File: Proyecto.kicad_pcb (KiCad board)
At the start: 2 copper layers, 108.2 x 65.5 mm, 54 parts, among them P1 CONN_01X03, P2 CONN_01X03, Q1 BC808-40, Q2 BC808-40, U1 MCP2515, U2 MCP2551-I/SN, U3 AMS1117, U4 ACS712, U5 ACS712, U6 AMS1117

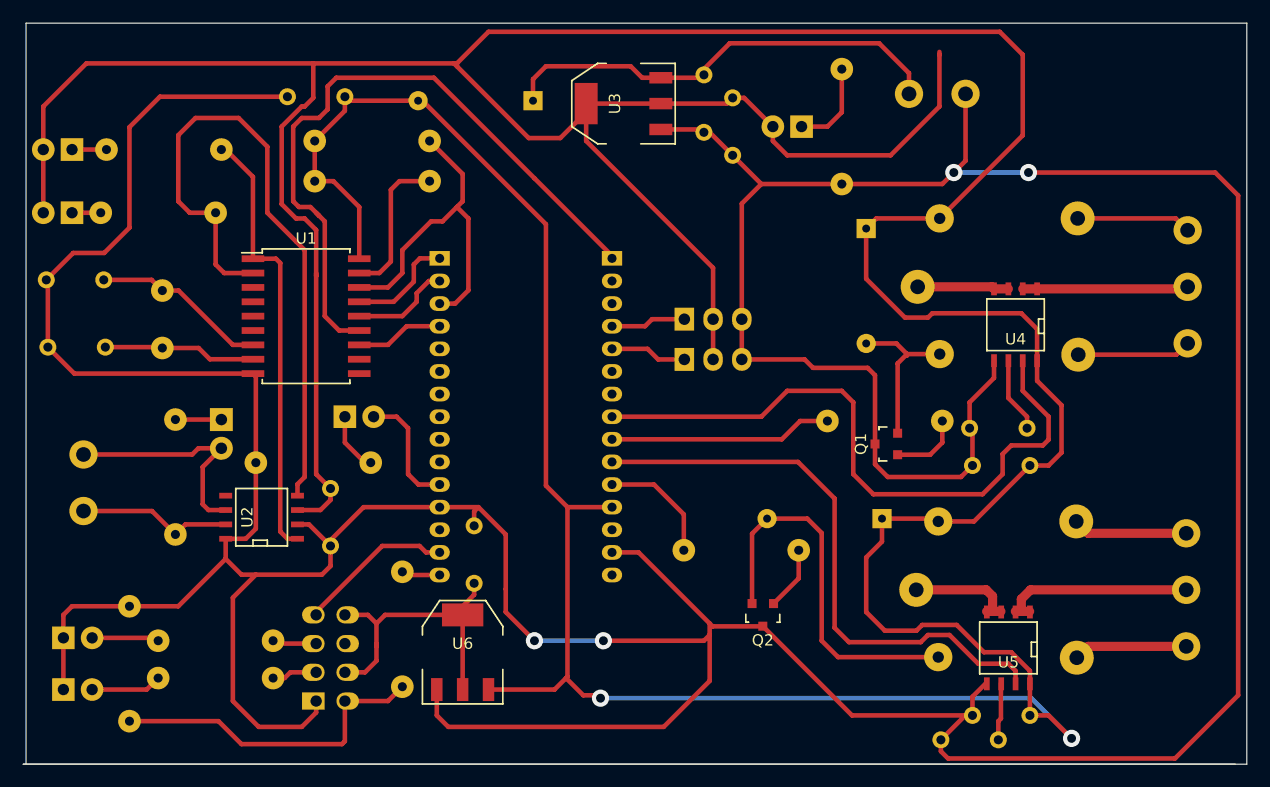
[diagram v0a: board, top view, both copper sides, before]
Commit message: fix
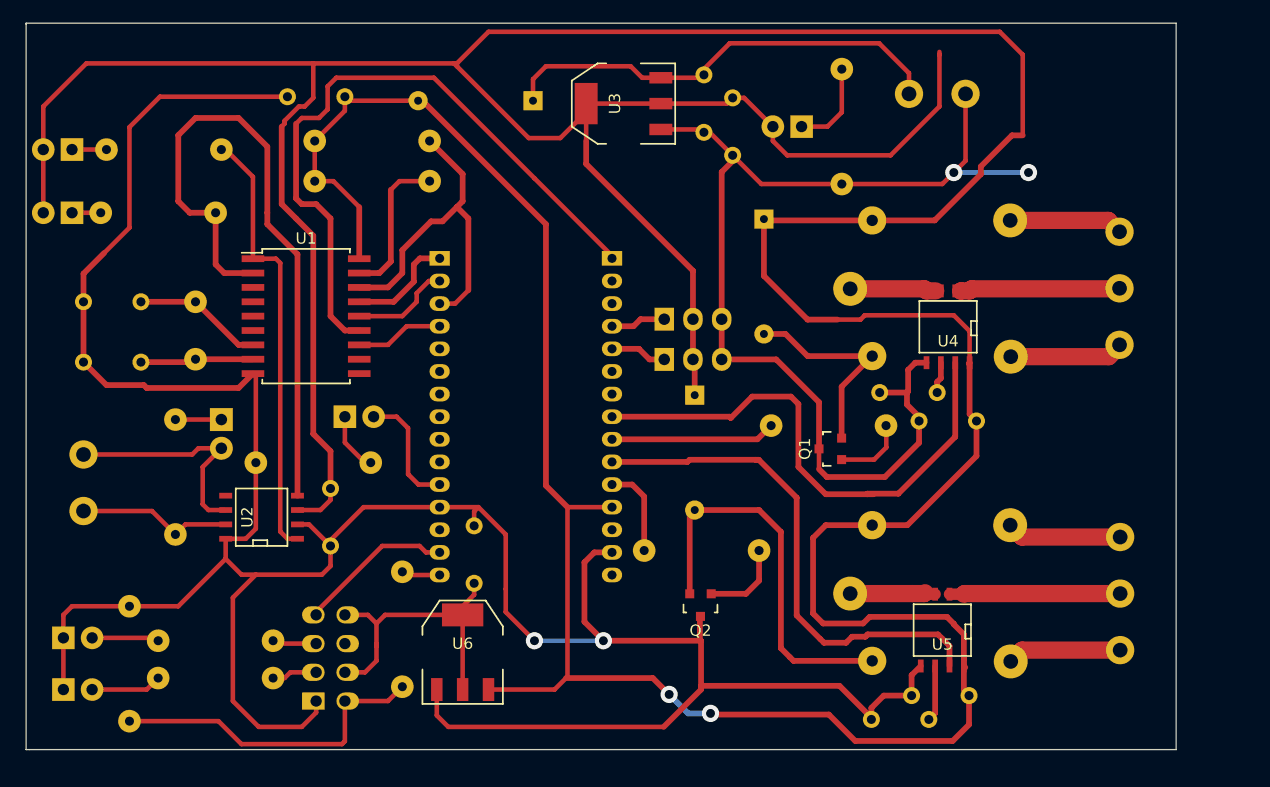
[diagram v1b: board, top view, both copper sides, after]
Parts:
- moved D3 19.8 mm to (117.6, 80.6), turned to 270 degrees
- moved D2 9.08 mm to (123.7, 65.1)
- moved CFilter1 8.55 mm to (136.4, 80.4)
- moved CFliter1 6.41 mm to (135.7, 109.3)
- moved C11 6.15 mm to (139.9, 82.9)
- moved U5 6.05 mm to (139.4, 101.4)
- moved P1 6.02 mm to (155.1, 71.2)
- moved Relay1 5.97 mm to (131.3, 71.2)
- moved U4 5.97 mm to (140.0, 74.6)
- moved P2 5.85 mm to (155.2, 98.2)
- moved Relay2 5.85 mm to (131.3, 98.2)
- moved C4 5.66 mm to (139.3, 107.2)
- moved Q2 5.58 mm to (118.1, 99.2)
- moved R3 4.99 mm to (129.4, 83.3)
- moved Q1 4.97 mm to (129.5, 85.4)
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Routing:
- net GND: track 454.3 -> 345.6 mm
- net Net-(P1-Pad2): track 14.7 -> 28.8 mm
- net /AC1: track 58.0 -> 47.2 mm
- net /AC2: track 51.7 -> 45.2 mm
- net /R2: track 19.7 -> 14.6 mm
- net Net-(D2-Pad2): track 14.5 -> 18.8 mm
- net Net-(C9-Pad1): track 15.6 -> 11.5 mm
- net Net-(CFilter1-Pad1): track 6.65 -> 2.78 mm
- net Net-(C8-Pad1): track 13.5 -> 10.0 mm
- net /R1: track 10.6 -> 8.06 mm
- net Net-(P2-Pad2): track 17.3 -> 15.1 mm
- net /PIN24: track 6.65 -> 4.88 mm
- net /PIN23: track 6.79 -> 5.01 mm
- net Net-(Q2-Pad1): track 5.64 -> 7.38 mm
- net Net-(P2-Pad1): track 10.2 -> 11.6 mm
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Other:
- board size 108.2 x 65.5 mm -> 101.7 x 64.2 mm
